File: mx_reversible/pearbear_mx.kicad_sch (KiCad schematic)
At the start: 20 parts, among them J1 rj11, SW1 SW_Push, SW10 SW_Push, SW11 SW_Push, SW12 SW_Push, SW13 SW_Push, SW14 SW_Push, SW15 SW_Push, SW16 SW_Push, SW17 SW_Push, SW2 SW_Push, SW3 SW_Push, SW4 SW_Push, SW5 SW_Push, SW6 SW_Push, SW7 SW_Push, SW8 SW_Push, SW9 SW_Push, U1 ProMicro-kbd-rev

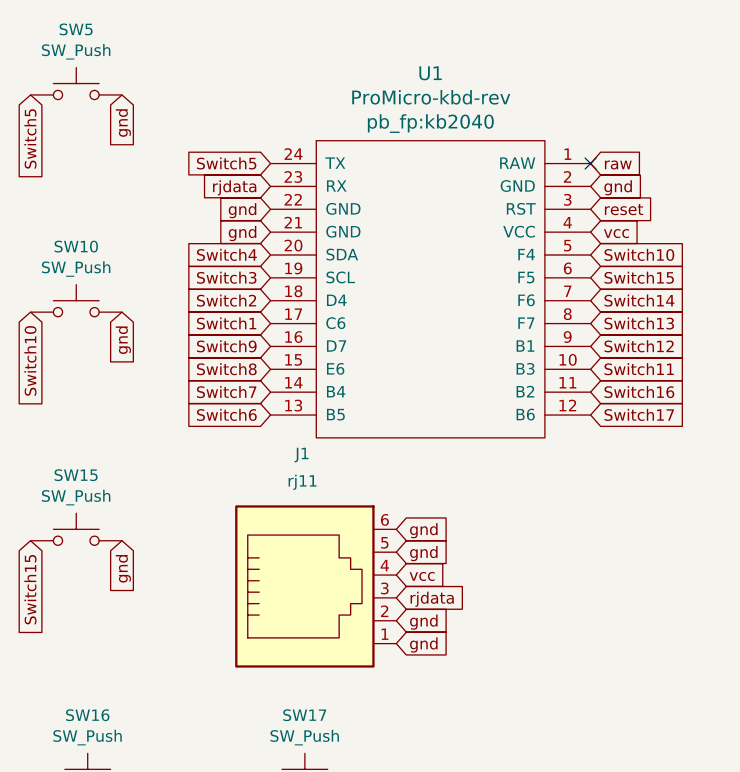
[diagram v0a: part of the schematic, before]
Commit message: hi
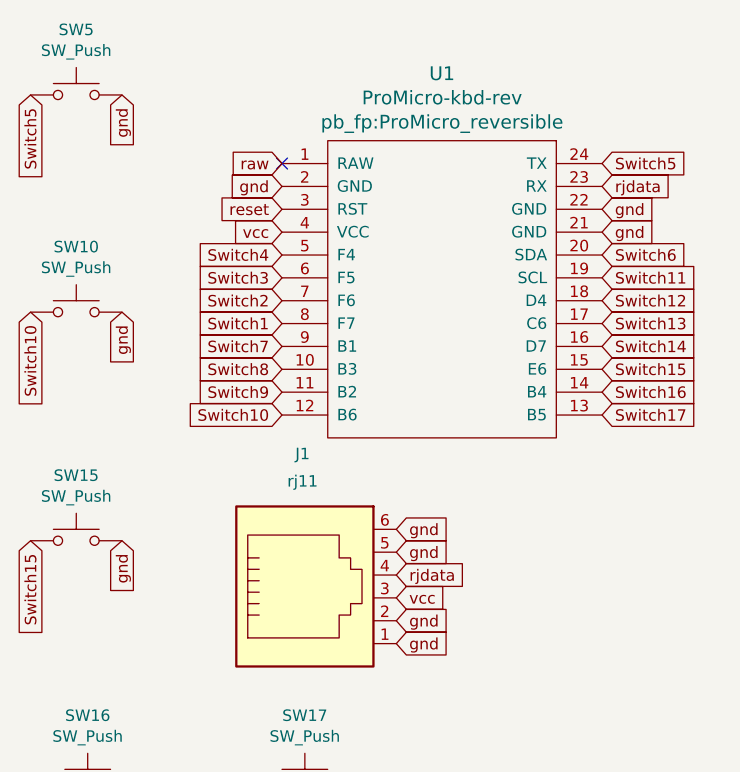
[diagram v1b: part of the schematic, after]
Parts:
- J1: footprint pb_fp:RJ11_6P6C -> pb_fp:RJ11_6P6C_reversible
- SW1, SW10, SW11, SW12, SW13, SW14, SW15, SW16, SW17, SW2, SW3, SW4, SW5, SW6, SW7, SW8, SW9: footprint pb_fp:SW_Cherry_MX -> pb_fp:SW_Cherry_MX_reversible
- U1: footprint pb_fp:kb2040 -> pb_fp:ProMicro_reversible
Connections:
- net Switch1: now also U1.8 (F7); no longer U1.17 (C6)
- net Switch10: now also U1.12 (B6); no longer U1.5 (F4)
- net Switch11: now also U1.19 (SCL); no longer U1.10 (B3)
- net Switch12: now also U1.18 (D4); no longer U1.9 (B1)
- net Switch13: now also U1.17 (C6); no longer U1.8 (F7)
- net Switch14: now also U1.16 (D7); no longer U1.7 (F6)
- net Switch15: now also U1.15 (E6); no longer U1.6 (F5)
- net Switch16: now also U1.14 (B4); no longer U1.11 (B2)
- net Switch17: now also U1.13 (B5); no longer U1.12 (B6)
- net Switch2: now also U1.7 (F6); no longer U1.18 (D4)
- net Switch3: now also U1.6 (F5); no longer U1.19 (SCL)
- net Switch4: now also U1.5 (F4); no longer U1.20 (SDA)
- net Switch6: now also U1.20 (SDA); no longer U1.13 (B5)
- net Switch7: now also U1.9 (B1); no longer U1.14 (B4)
- net Switch8: now also U1.10 (B3); no longer U1.15 (E6)
- net Switch9: now also U1.11 (B2); no longer U1.16 (D7)
- net rjdata: now also J1.4; no longer J1.3
- net vcc: now also J1.3; no longer J1.4
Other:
- moved on the sheet: U1
